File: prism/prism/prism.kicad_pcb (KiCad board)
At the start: 2 copper layers, 62 x 100 mm, 11 parts, among them J1 in1, J2 in2, J3 in3, J4 in4, J5 out1, J6 out2, J7 out3, J8 out4, SW1 Rotary_Encoder_Switch, U1 MCP4728

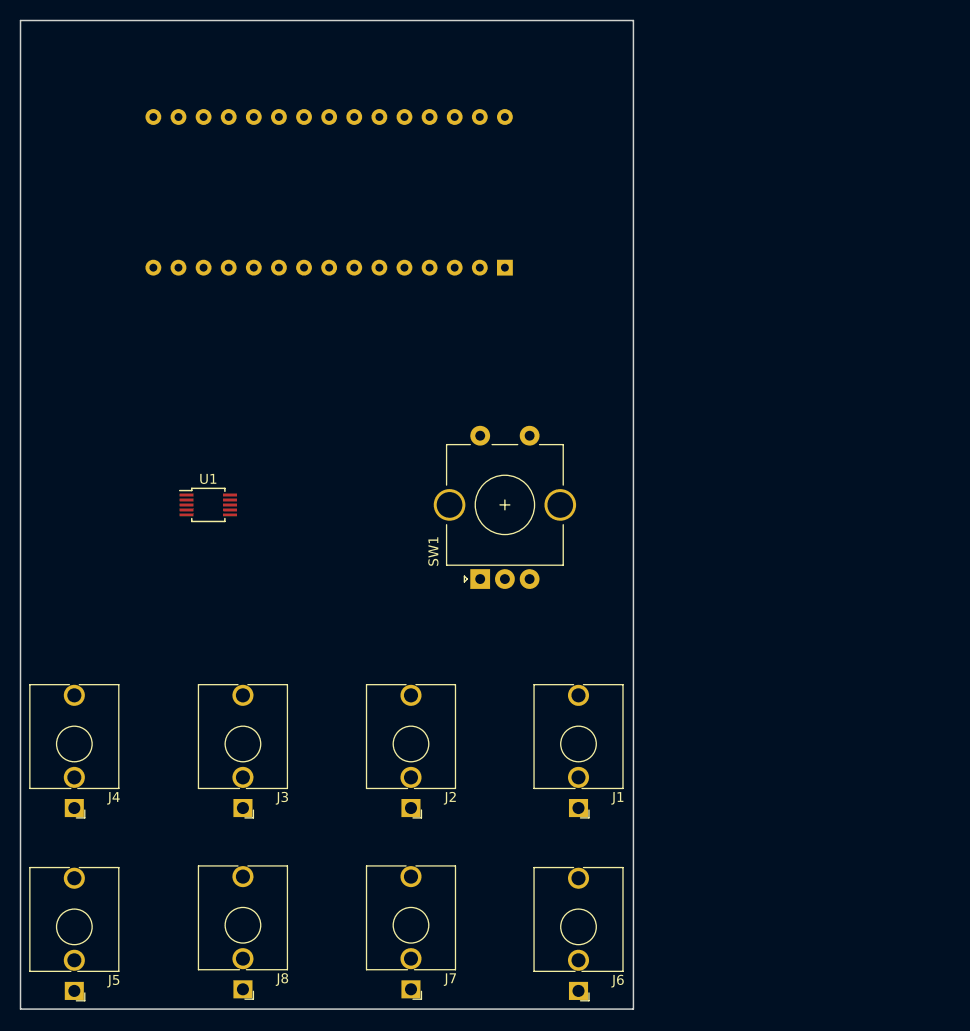
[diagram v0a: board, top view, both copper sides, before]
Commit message: All kinds of stuff
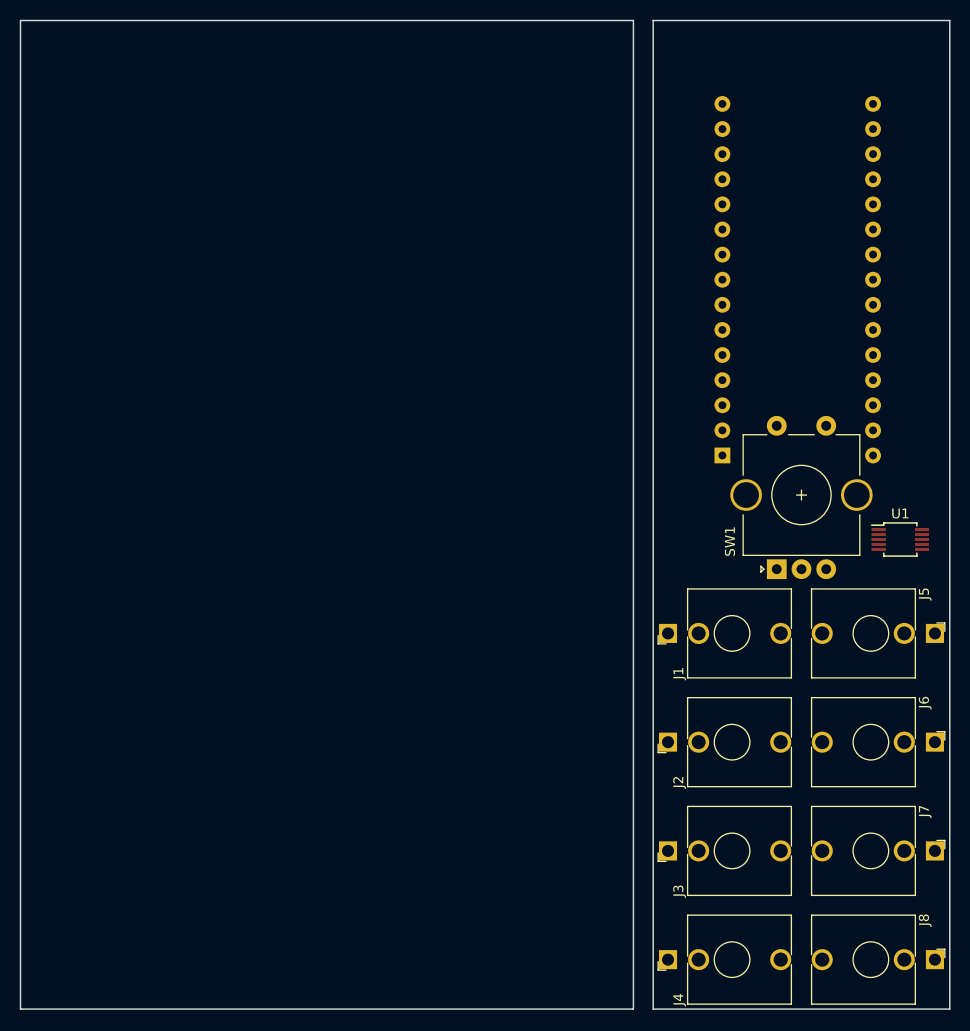
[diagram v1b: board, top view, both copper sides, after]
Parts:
- moved J5 94.3 mm to (181.5, 90.5), turned to 270 degrees
- moved U1 70.1 mm to (178.0, 81.0)
- moved J8 70.1 mm to (181.5, 123.5), turned to 270 degrees
- moved J4 62.0 mm to (154.5, 123.5), turned to 90 degrees
- moved J7 54.8 mm to (181.5, 112.5), turned to 270 degrees
- moved J6 44.0 mm to (181.5, 101.5), turned to 270 degrees
- moved J3 43.2 mm to (154.5, 112.5), turned to 90 degrees
- moved SW1 30.0 mm to (165.5, 84.0)
- moved A1 29.1 mm to (160.0, 72.5), turned to 0 degrees
- moved J2 26.8 mm to (154.5, 101.5), turned to 90 degrees
- moved J1 19.8 mm to (154.5, 90.5), turned to 90 degrees
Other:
- board size 62 x 100 mm -> 94 x 100 mm
